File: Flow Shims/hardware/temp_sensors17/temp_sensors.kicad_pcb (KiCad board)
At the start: 2 copper layers, 6 x 113 mm, 36 parts, among them J1 Conn_01x03, U10 TMP1826NG, U11 TMP1826NG, U12 TMP1826NG, U13 TMP1826NG, U14 TMP1826NG, U15 TMP1826NG, U16 TMP1826NG, U17 TMP1826NG, U18 TMP1826NG, U2 TMP1826NG, U3 TMP1826NG, U4 TMP1826NG, U5 TMP1826NG, U6 TMP1826NG, U7 TMP1826NG, U8 TMP1826NG, U9 TMP1826NG

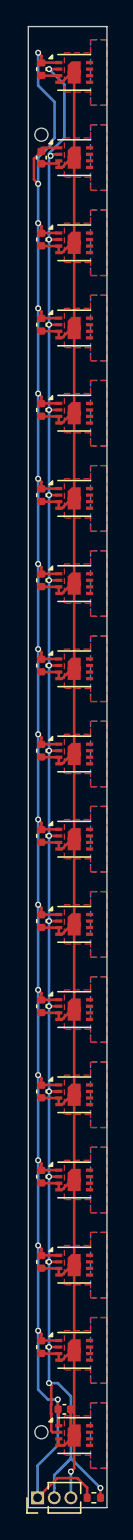
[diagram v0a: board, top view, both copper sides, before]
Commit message: All boards DRC/ERC clean
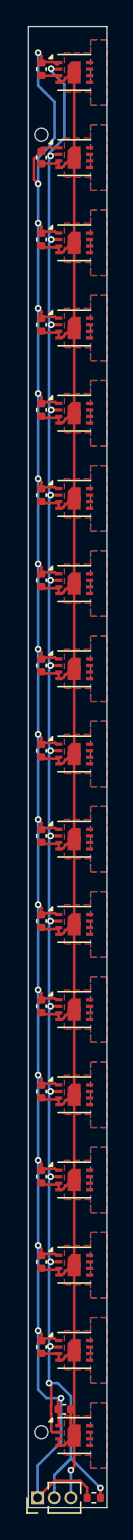
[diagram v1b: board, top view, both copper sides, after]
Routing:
- net +3.3V: track 154.5 -> 156.6 mm
- net GND: track 162.4 -> 163.6 mm
